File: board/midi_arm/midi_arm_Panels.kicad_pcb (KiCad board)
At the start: 2 copper layers, 100 x 100 mm, 75 parts, among them J1 Conn_01x02_Pin, J2 Conn_01x02_Pin, J3 Conn_01x10_Pin, J4 RJ45, J5 Conn_01x03_Pin, J6 Conn_01x03_Pin, J7 Conn_01x03_Pin, U6 6DOF_6050

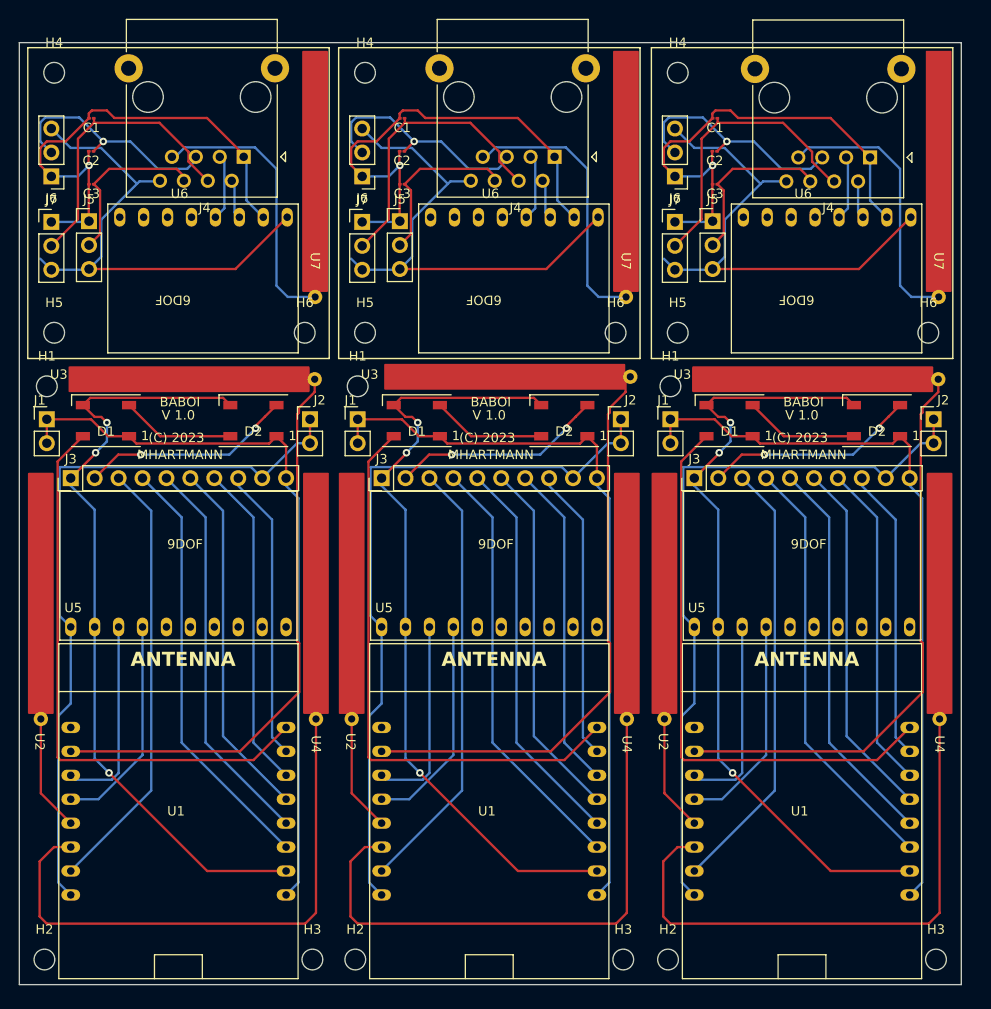
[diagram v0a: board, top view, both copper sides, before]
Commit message: BABOI 2.0 Board
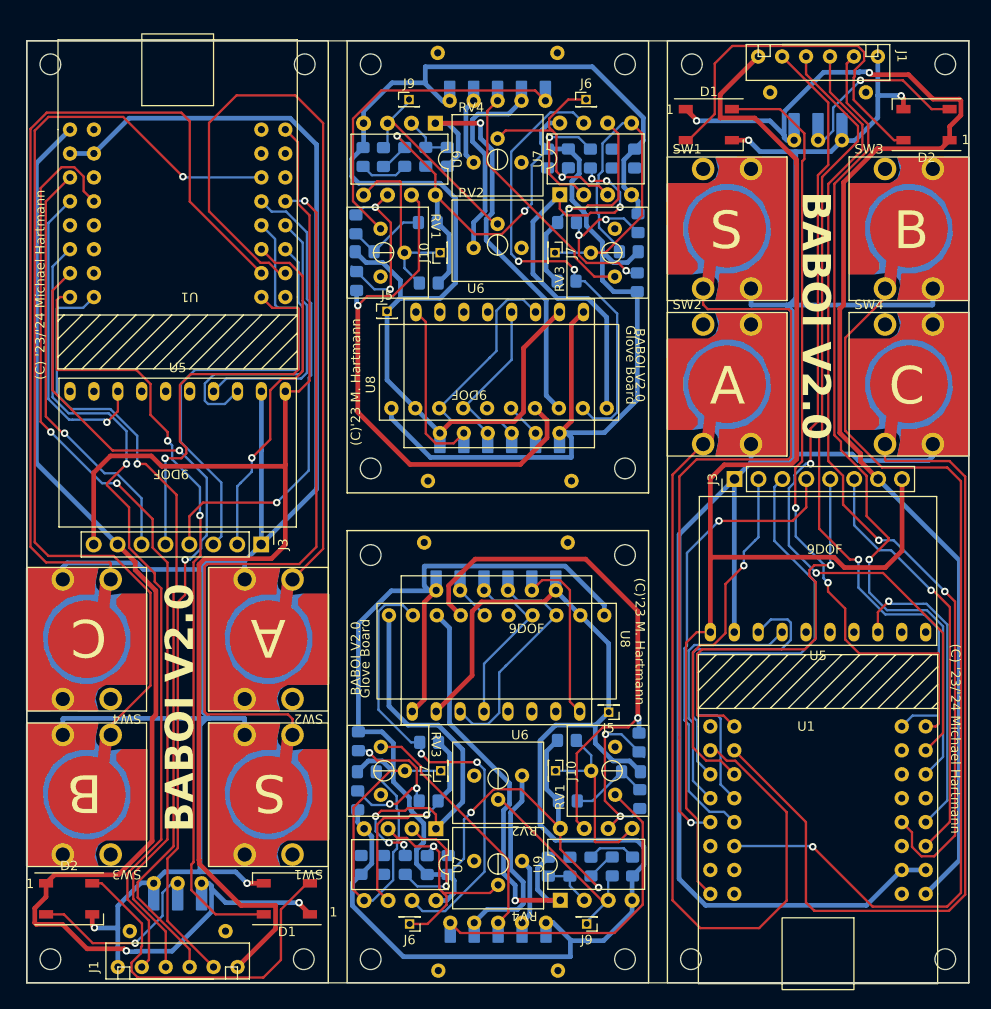
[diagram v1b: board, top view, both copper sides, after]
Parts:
- removed C1 (x3), C2 (x3), C3 (x3): 100nF, Capacitor_SMD:C_01005_0402Metric
- removed the D1 at (165.4, 65.1)
- removed the D1 at (132.2, 65.1)
- removed the D1 at (99.2, 65.1)
- removed the D2 at (114.8, 65.1)
- removed the D2 at (181.1, 65.1)
- removed the D2 at (147.8, 65.1)
- removed the H1 at (125.9, 61.5)
- removed the H1 at (92.9, 61.5)
- removed the H1 at (159.1, 61.5)
- removed the H2 at (92.7, 122.3)
- removed the H2 at (125.7, 122.3)
- removed the H2 at (158.9, 122.3)
- removed the H3 at (121.1, 122.3)
- removed the H3 at (187.3, 122.3)
- removed the H3 at (154.1, 122.3)
- removed the H4 at (126.7, 28.2)
- removed the H4 at (93.7, 28.2)
- removed the H4 at (159.9, 28.2)
- removed the H5 at (159.9, 55.8)
- removed the H5 at (93.7, 55.8)
- removed the H5 at (126.7, 55.8)
- removed the H6 at (120.3, 55.8)
- removed the H6 at (153.3, 55.8)
- removed the H6 at (186.5, 55.8)
- removed the J1 at (159.1, 65.0)
- removed the J1 at (92.9, 65.0)
- removed the J1 at (125.9, 65.0)
- removed the J2 at (120.9, 65.0)
- removed the J2 at (187.1, 65.0)
- removed the J2 at (153.9, 65.0)
- removed the J3 at (95.5, 71.2)
- removed the J3 at (161.7, 71.2)
- removed the J3 at (128.5, 71.2)
- removed the J4 at (113.8, 37.1)
- removed the J4 at (146.8, 37.1)
- removed the J4 at (180.3, 37.2)
- removed the J5 at (97.4, 44.0)
- removed the J5 at (163.6, 44.0)
- removed the J5 at (130.4, 44.0)
- removed the J6 at (93.4, 39.2)
- removed the J6 at (126.4, 39.2)
- removed the J6 at (159.6, 39.2)
- removed the J7 at (126.4, 44.0)
- removed the J7 at (93.4, 44.0)
- removed the J7 at (159.6, 44.0)
- removed the U1 at (139.9, 106.6)
- removed the U1 at (173.1, 106.6)
- removed the U1 at (106.9, 106.6)
- removed U2 (x3), U3 (x3), U4 (x3): ~, midi_arm:TOUCH_BAR
- removed the U5 at (106.9, 87.0)
- removed the U5 at (173.1, 87.0)
- removed the U5 at (139.9, 87.0)
- removed the U6 at (107.0, 43.5)
- removed the U6 at (173.2, 43.5)
- removed the U6 at (140.0, 43.5)
- removed the U7 at (121.4, 59.6)
- removed the U7 at (187.6, 59.6)
- removed the U7 at (154.4, 59.6)
- added D1: WS2812B, LED_SMD:LED_WS2812B_PLCC4_5.0x5.0mm_P3.2mm, F.Cu at (118.4, 115.9)
- added D1: WS2812B, LED_SMD:LED_WS2812B_PLCC4_5.0x5.0mm_P3.2mm, F.Cu at (163.2, 33.7)
- added D2: WS2812B, LED_SMD:LED_WS2812B_PLCC4_5.0x5.0mm_P3.2mm, F.Cu at (186.3, 33.7)
- added D2: WS2812B, LED_SMD:LED_WS2812B_PLCC4_5.0x5.0mm_P3.2mm, F.Cu at (95.3, 115.9)
- added H1: MountingHole, MountingHole:MountingHole_2.2mm_M2, F.Cu at (161.4, 27.3)
- added H1: MountingHole, MountingHole:MountingHole_2.2mm_M2, F.Cu at (120.2, 122.3)
- added H2: MountingHole, MountingHole:MountingHole_2.2mm_M2, F.Cu at (93.3, 122.3)
- added H2: MountingHole, MountingHole:MountingHole_2.2mm_M2, F.Cu at (188.3, 27.3)
- added H3: MountingHole, MountingHole:MountingHole_2.2mm_M2, F.Cu at (120.3, 27.3)
- added H3: MountingHole, MountingHole:MountingHole_2.2mm_M2, F.Cu at (161.3, 122.3)
- added H4: MountingHole, MountingHole:MountingHole_2.2mm_M2, F.Cu at (93.3, 27.3)
- added H4: MountingHole, MountingHole:MountingHole_2.2mm_M2, F.Cu at (188.3, 122.3)
- added H5: MountingHole, MountingHole:MountingHole_2.2mm_M2, F.Cu at (127.3, 79.4)
- added H5: MountingHole, MountingHole:MountingHole_2.2mm_M2, F.Cu at (154.3, 70.2)
- added H6: MountingHole, MountingHole:MountingHole_2.2mm_M2, F.Cu at (127.3, 70.2)
- added H6: MountingHole, MountingHole:MountingHole_2.2mm_M2, F.Cu at (154.3, 79.4)
- added H7: MountingHole, MountingHole:MountingHole_2.2mm_M2, F.Cu at (127.3, 27.3)
- added H7: MountingHole, MountingHole:MountingHole_2.2mm_M2, F.Cu at (154.3, 122.3)
- added H8: MountingHole, MountingHole:MountingHole_2.2mm_M2, F.Cu at (154.3, 27.3)
- added H8: MountingHole, MountingHole:MountingHole_2.2mm_M2, F.Cu at (127.3, 122.3)
- added J1: Conn_01x06_Pin, GPB_Footprints:JST_1x6_2.54, F.Cu at (100.5, 123.1)
- added J1: Conn_01x06_Pin, GPB_Footprints:JST_1x6_2.54, F.Cu at (181.1, 26.5)
- added J10: Conn_01x01_Pin, Connector_PinHeader_1.27mm:PinHeader_1x01_P1.27mm_Vertical, F.Cu at (146.9, 102.3)
- added J10: Conn_01x01_Pin, Connector_PinHeader_1.27mm:PinHeader_1x01_P1.27mm_Vertical, F.Cu at (134.7, 47.3)
- added J2: Conn_01x03_Pin, midi_arm:LED_conn, B.Cu at (182.4, 35.4)
- added J2: Conn_01x03_Pin, midi_arm:LED_conn, B.Cu at (99.2, 114.2)
- added J3: Conn_01x08_Pin, Connector_PinHeader_2.54mm:PinHeader_1x08_P2.54mm_Vertical, F.Cu at (165.9, 71.3)
- added J3: Conn_01x08_Pin, Connector_PinHeader_2.54mm:PinHeader_1x08_P2.54mm_Vertical, F.Cu at (115.7, 78.3)
- added J4: Conn_01x05_Pin, GPB_Footprints:JST_1x5_2.54_cablepad, B.Cu at (145.8, 31.2)
- added J4: Conn_01x05_Pin, GPB_Footprints:JST_1x5_2.54_cablepad, B.Cu at (135.8, 118.4)
- added J5: Conn_01x01_Pin, Connector_PinHeader_1.27mm:PinHeader_1x01_P1.27mm_Vertical, F.Cu at (152.6, 96.1)
- added J5: Conn_01x01_Pin, Connector_PinHeader_1.27mm:PinHeader_1x01_P1.27mm_Vertical, F.Cu at (129.0, 53.5)
- added J6: Conn_01x01_Pin, Connector_PinHeader_1.27mm:PinHeader_1x01_P1.27mm_Vertical, F.Cu at (131.4, 118.6)
- added J6: Conn_01x01_Pin, Connector_PinHeader_1.27mm:PinHeader_1x01_P1.27mm_Vertical, F.Cu at (150.2, 31.0)
- added J7: Conn_01x01_Pin, Connector_PinHeader_1.27mm:PinHeader_1x01_P1.27mm_Vertical, F.Cu at (134.7, 102.3)
- added J7: Conn_01x01_Pin, Connector_PinHeader_1.27mm:PinHeader_1x01_P1.27mm_Vertical, F.Cu at (146.9, 47.3)
- added J8: Conn_01x06_Pin, GPB_Footprints:JST_1x6_2.54_cablepad, B.Cu at (147.0, 83.2)
- added J8: Conn_01x06_Pin, GPB_Footprints:JST_1x6_2.54_cablepad, B.Cu at (134.6, 66.4)
- added J9: Conn_01x01_Pin, Connector_PinHeader_1.27mm:PinHeader_1x01_P1.27mm_Vertical, F.Cu at (131.4, 31.0)
- added J9: Conn_01x01_Pin, Connector_PinHeader_1.27mm:PinHeader_1x01_P1.27mm_Vertical, F.Cu at (150.2, 118.6)
- added R1: 2.4k, Resistor_SMD:R_0805_2012Metric_Pad1.20x1.40mm_HandSolder, B.Cu at (135.5, 112.3)
- added R1: 2.4k, Resistor_SMD:R_0805_2012Metric_Pad1.20x1.40mm_HandSolder, B.Cu at (146.1, 37.3)
- added R10: 24k, Resistor_SMD:R_0805_2012Metric_Pad1.20x1.40mm_HandSolder, B.Cu at (148.1, 50.3)
- added R10: 24k, Resistor_SMD:R_0805_2012Metric_Pad1.20x1.40mm_HandSolder, B.Cu at (133.5, 99.3)
- added R11: 2.4k, Resistor_SMD:R_0805_2012Metric_Pad1.20x1.40mm_HandSolder, B.Cu at (130.9, 37.1)
- added R11: 2.4k, Resistor_SMD:R_0805_2012Metric_Pad1.20x1.40mm_HandSolder, B.Cu at (150.7, 112.5)
- added R12: 2.4k, Resistor_SMD:R_0805_2012Metric_Pad1.20x1.40mm_HandSolder, B.Cu at (128.7, 37.1)
- added R12: 2.4k, Resistor_SMD:R_0805_2012Metric_Pad1.20x1.40mm_HandSolder, B.Cu at (152.9, 112.5)
- added R13: 2.4k, Resistor_SMD:R_0805_2012Metric_Pad1.20x1.40mm_HandSolder, B.Cu at (155.1, 112.5)
- added R13: 2.4k, Resistor_SMD:R_0805_2012Metric_Pad1.20x1.40mm_HandSolder, B.Cu at (126.5, 37.1)
- added R14: 2.4k, Resistor_SMD:R_0805_2012Metric_Pad1.20x1.40mm_HandSolder, B.Cu at (133.2, 37.1)
- added R14: 2.4k, Resistor_SMD:R_0805_2012Metric_Pad1.20x1.40mm_HandSolder, B.Cu at (148.4, 112.5)
- added R15: 24k, Resistor_SMD:R_0805_2012Metric_Pad1.20x1.40mm_HandSolder, B.Cu at (146.2, 112.5)
- added R15: 24k, Resistor_SMD:R_0805_2012Metric_Pad1.20x1.40mm_HandSolder, B.Cu at (135.4, 37.1)
- added R16: 2.4k, Resistor_SMD:R_0805_2012Metric_Pad1.20x1.40mm_HandSolder, B.Cu at (133.4, 44.1)
- added R16: 2.4k, Resistor_SMD:R_0805_2012Metric_Pad1.20x1.40mm_HandSolder, B.Cu at (148.2, 105.5)
- added R17: 2.4k, Resistor_SMD:R_0805_2012Metric_Pad1.20x1.40mm_HandSolder, B.Cu at (148.1, 99.1)
- added R17: 2.4k, Resistor_SMD:R_0805_2012Metric_Pad1.20x1.40mm_HandSolder, B.Cu at (133.5, 50.5)
- added R18: 2.4k, Resistor_SMD:R_0805_2012Metric_Pad1.20x1.40mm_HandSolder, B.Cu at (154.9, 102.4)
- added R18: 2.4k, Resistor_SMD:R_0805_2012Metric_Pad1.20x1.40mm_HandSolder, B.Cu at (126.7, 47.2)
- added R19: 2.4k, Resistor_SMD:R_0805_2012Metric_Pad1.20x1.40mm_HandSolder, B.Cu at (155.9, 105.3)
- added R19: 2.4k, Resistor_SMD:R_0805_2012Metric_Pad1.20x1.40mm_HandSolder, B.Cu at (125.7, 44.3)
- added R2: 2.4k, Resistor_SMD:R_0805_2012Metric_Pad1.20x1.40mm_HandSolder, B.Cu at (155.3, 37.3)
- added R2: 2.4k, Resistor_SMD:R_0805_2012Metric_Pad1.20x1.40mm_HandSolder, B.Cu at (126.3, 112.3)
- added R20: 24k, Resistor_SMD:R_0805_2012Metric_Pad1.20x1.40mm_HandSolder, B.Cu at (155.8, 99.3)
- added R20: 24k, Resistor_SMD:R_0805_2012Metric_Pad1.20x1.40mm_HandSolder, B.Cu at (125.8, 50.3)
- added R3: 2.4k, Resistor_SMD:R_0805_2012Metric_Pad1.20x1.40mm_HandSolder, B.Cu at (148.3, 37.3)
- added R3: 2.4k, Resistor_SMD:R_0805_2012Metric_Pad1.20x1.40mm_HandSolder, B.Cu at (133.3, 112.3)
- added R4: 2.4k, Resistor_SMD:R_0805_2012Metric_Pad1.20x1.40mm_HandSolder, B.Cu at (152.9, 37.3)
- added R4: 2.4k, Resistor_SMD:R_0805_2012Metric_Pad1.20x1.40mm_HandSolder, B.Cu at (128.7, 112.3)
- added R5: 24k, Resistor_SMD:R_0805_2012Metric_Pad1.20x1.40mm_HandSolder, B.Cu at (131.0, 112.3)
- added R5: 24k, Resistor_SMD:R_0805_2012Metric_Pad1.20x1.40mm_HandSolder, B.Cu at (150.6, 37.3)
- added R6: 2.4k, Resistor_SMD:R_0805_2012Metric_Pad1.20x1.40mm_HandSolder, B.Cu at (155.6, 50.4)
- added R6: 2.4k, Resistor_SMD:R_0805_2012Metric_Pad1.20x1.40mm_HandSolder, B.Cu at (126.0, 99.2)
- added R7: 2.4k, Resistor_SMD:R_0805_2012Metric_Pad1.20x1.40mm_HandSolder, B.Cu at (154.7, 47.2)
- added R7: 2.4k, Resistor_SMD:R_0805_2012Metric_Pad1.20x1.40mm_HandSolder, B.Cu at (126.9, 102.4)
- added R8: 2.4k, Resistor_SMD:R_0805_2012Metric_Pad1.20x1.40mm_HandSolder, B.Cu at (125.9, 105.4)
- added R8: 2.4k, Resistor_SMD:R_0805_2012Metric_Pad1.20x1.40mm_HandSolder, B.Cu at (155.7, 44.2)
- added R9: 2.4k, Resistor_SMD:R_0805_2012Metric_Pad1.20x1.40mm_HandSolder, B.Cu at (148.1, 44.1)
- added R9: 2.4k, Resistor_SMD:R_0805_2012Metric_Pad1.20x1.40mm_HandSolder, B.Cu at (133.5, 105.5)
- added RV1: R_Potentiometer_Small, midi_arm:pot_9.5x9.5, F.Cu at (137.2, 47.3)
- added RV1: R_Potentiometer_Small, midi_arm:pot_9.5x9.5, F.Cu at (144.4, 102.3)
- added RV2: R_Potentiometer_Small, midi_arm:pot_9.5x9.5, F.Cu at (140.8, 111.7)
- added RV2: R_Potentiometer_Small, midi_arm:pot_9.5x9.5, F.Cu at (140.8, 37.9)
- added RV3: R_Potentiometer_Small, midi_arm:pot_9.5x9.5, F.Cu at (137.3, 102.3)
- added RV3: R_Potentiometer_Small, midi_arm:pot_9.5x9.5, F.Cu at (144.3, 47.3)
- added RV4: R_Potentiometer_Small, midi_arm:pot_9.5x9.5, F.Cu at (140.8, 120.8)
- added RV4: R_Potentiometer_Small, midi_arm:pot_9.5x9.5, F.Cu at (140.8, 28.8)
- added SW1: SW_MEC_5E, GPB_Footprints:switch_Touchpad, F.Cu at (162.6, 38.4)
- added SW1: SW_MEC_5E, GPB_Footprints:switch_Touchpad, F.Cu at (119.0, 111.2)
- added SW2: SW_MEC_5E, GPB_Footprints:switch_Touchpad, F.Cu at (162.6, 54.9)
- added SW2: SW_MEC_5E, GPB_Footprints:switch_Touchpad, F.Cu at (119.0, 94.7)
- added SW3: SW_MEC_5E, GPB_Footprints:switch_Touchpad, F.Cu at (99.7, 111.2)
- added SW3: SW_MEC_5E, GPB_Footprints:switch_Touchpad, F.Cu at (181.9, 38.4)
- added SW4: SW_MEC_5E, GPB_Footprints:switch_Touchpad, F.Cu at (99.7, 94.7)
- added SW4: SW_MEC_5E, GPB_Footprints:switch_Touchpad, F.Cu at (181.9, 54.9)
- added U1: ~, GPB_Footprints:ESP32_S2_Wemos_Mini, F.Cu at (163.4, 97.6)
- added U1: ~, GPB_Footprints:ESP32_S2_Wemos_Mini, F.Cu at (118.2, 52.0)
- added U5: ~, midi_arm:9250_MOD, F.Cu at (174.8, 87.6)
- added U5: ~, midi_arm:9250_MOD, F.Cu at (106.8, 62.0)
- added U6: 6DOF_6050, midi_arm:6050_MOD, F.Cu at (138.5, 53.6)
- added U6: 6DOF_6050, midi_arm:6050_MOD, F.Cu at (143.1, 96.0)
- added U7: ~, Package_DIP:DIP-8_W7.62mm, F.Cu at (147.4, 41.2)
- added U7: ~, Package_DIP:DIP-8_W7.62mm, F.Cu at (134.2, 108.4)
- added U8: ~, midi_arm:ADS1115_mod, F.Cu at (124.4, 63.8)
- added U8: ~, midi_arm:ADS1115_mod, F.Cu at (157.2, 85.8)
- added U9: ~, Package_DIP:DIP-8_W7.62mm, F.Cu at (147.4, 116.0)
- added U9: ~, Package_DIP:DIP-8_W7.62mm, F.Cu at (134.2, 33.6)
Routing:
- net /VCC_3V3: track 0.00 -> 272.5 mm
- net /GLOVE_VCC: track 0.00 -> 268.9 mm, vias 0 -> 4
- net GND2: track 0.00 -> 264.3 mm
- net Net-(J2-Pin_1): track 234.4 -> 0.00 mm
- net Net-(U1-GPIO_10): track 0.00 -> 204.7 mm, vias 0 -> 2
- net /EXT_SCL: track 0.00 -> 202.2 mm, vias 0 -> 4
- net Net-(U1-GPIO_2): track 0.00 -> 185.2 mm
- net Net-(U1-3): track 182.8 -> 0.00 mm
- net Net-(U1-11): track 181.5 -> 0.00 mm
- net /ALERT: track 0.00 -> 178.8 mm, vias 0 -> 4
- net /INT: track 0.00 -> 177.4 mm, vias 0 -> 2
- net /EXT_SDA: track 0.00 -> 173.1 mm, vias 0 -> 2
- net Net-(U1-GPIO_3): track 0.00 -> 169.1 mm
- net Net-(J5-Pin_3): track 165.3 -> 0.00 mm
- net Net-(J5-Pin_1): track 157.7 -> 0.00 mm, vias 3 -> 0
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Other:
- board text added: "(C) '23/'24 Michael Hartmann"
- board text added: "(C)'23 M. Hartmann"
- board text added: "A"
- board text added: "B"
- board text added: "BABOI V2.0"
- board text added: "C"
- board text added: "Glove Board"
- board text added: "S"
- board text removed: "(C) 2023"
- board text removed: "BABOI"
- board text removed: "MHARTMANN"
- board text removed: "V 1.0"
